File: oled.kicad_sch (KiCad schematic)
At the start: 1 part, among them J15 HC-SR04 connector

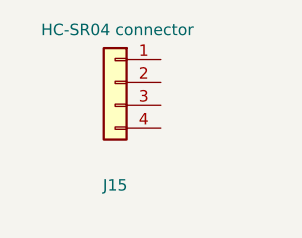
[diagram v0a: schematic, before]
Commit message: No Errors No Warnings
Some were excluded.
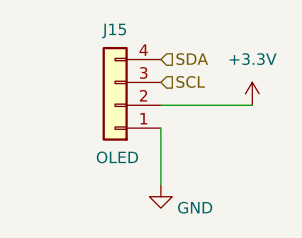
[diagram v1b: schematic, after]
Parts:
- J15: value HC-SR04 connector -> OLED; footprint Connector_PinHeader_2.54mm:PinHeader_1x04_P2.54mm_Vertical -> Connector_PinSocket_2.54mm:PinSocket_1x04_P2.54mm_Vertical
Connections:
- net GND: now reaches J15.1 (Pin_1)
- net +3.3V: now reaches J15.2 (Pin_2)
- net SCL: now reaches J15.3 (Pin_3)
- net SDA: now reaches J15.4 (Pin_4)
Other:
- moved on the sheet: J15
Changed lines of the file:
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@@
 	(generator_version "9.0")
 	(paper "A4")
+	(wire
+		(pts
+			(xy 134.62 80.01) (xy 134.62 86.36)
+		)
+		(stroke
+			(width 0)
+			(type default)
+		)
+	)
+	(wire
+		(pts
+			(xy 134.62 77.47) (xy 144.78 77.47)
+		)
+		(stroke
+			(width 0)
+			(type default)
+		)
+	)
+	(hierarchical_label "SDA"
+		(shape input)
+		(at 134.62 72.39 0)
+		(effects
+			(font
+				(size 1.27 1.27)
+			)
+			(justify left)
+		)
+	)
+	(hierarchical_label "SCL"
+		(shape input)
+		(at 134.62 74.93 0)
+		(effects
+			(font
+				(size 1.27 1.27)
+			)
+			(justify left)
+		)
+	)
+	(symbol
+		(lib_id "power:GND")
+		(at 134.62 86.36 0)
+		(unit 1)
+		(exclude_from_sim no)
+		(in_bom yes)
+		(on_board yes)
+		(dnp no)
+		(property "Reference" "#PWR0142"
+			(at 134.62 92.71 0)
+			(effects
+				(font
+					(size 1.27 1.27)
+				)
+				(hide yes)
+			)
+		)
+		(property "Value" "GND"
+			(at 138.43 88.9 0)
+			(effects
+				(font
+					(size 1.27 1.27)
+				)
+			)
+		)
+		(property "Footprint" ""
+			(at 134.62 86.36 0)
+			(effects
+				(font
+					(size 1.27 1.27)
+				)
+				(hide yes)
+			)
+		)
+		(property "Datasheet" ""
+			(at 134.62 86.36 0)
+			(effects
+				(font
+					(size 1.27 1.27)
+				)
+				(hide yes)
+			)
+		)
+		(property "Description" ""
+			(at 134.62 86.36 0)
+			(effects
+				(font
+					(size 1.27 1.27)
+				)
+				(hide yes)
+			)
+		)
+		(pin "1"
+		)
+		(instances
+			(project "Intro-to-CAD-2026"
+				(path "/c12dc015-e6cb-468c-8de4-269c3106de0e/77c9a60d-65a0-419f-902e-4b4a89f0d425"
+					(reference "#PWR0142")
+					(unit 1)
+				)
+			)
+		)
+	)
 	(symbol
 		(lib_id "Connector_Generic:Conn_01x04")
-		(at 129.54 74.93 0)
+		(at 129.54 77.47 180)
+		(unit 1)
+		(exclude_from_sim no)
+		(in_bom yes)
+		(on_board yes)
+		(dnp no)
+		(property "Reference" "J15"
+			(at 129.54 69.088 0)
+			(effects
+				(font
+					(size 1.27 1.27)
+				)
+			)
+		)
+		(property "Value" "OLED"
+			(at 129.794 83.312 0)
+			(effects
+				(font
+					(size 1.27 1.27)
+				)
+			)
+		)
+		(property "Footprint" "Connector_PinSocket_2.54mm:PinSocket_1x04_P2.54mm_Vertical"
+			(at 129.54 77.47 0)
+			(effects
+				(font
+					(size 1.27 1.27)
+				)
+				(hide yes)
+			)
+		)
+		(property "Datasheet" "https://www.robotshop.com/products/adeept-096in-oled-module-128x64-ssd1306-i2c-serial-self-luminous-display-4x?srsltid=AfmBOopotbcFOdiYSAv3nbip_y2fRyMvjxpTrSpnZLL8r5jh1ATbT-r4"
+			(at 129.54 77.47 0)
+			(effects
+				(font
+					(size 1.27 1.27)
+				)
+				(hide yes)
+			)
+		)
+		(property "Description" "Generic connector, single row, 01x04, script generated (kicad-library-utils/schlib/autogen/connector/)"
+			(at 129.54 77.47 0)
+			(effects
+				(font
+					(size 1.27 1.27)
+				)
+				(hide yes)
+			)
+		)
+		(pin "4"
+		)
+		(pin "1"
+		)
+		(pin "2"
+		)
+		(pin "3"
+		)
+		(instances
+			(project "Intro-to-CAD-2026"
+				(path "/c12dc015-e6cb-468c-8de4-269c3106de0e/77c9a60d-65a0-419f-902e-4b4a89f0d425"
+					(reference "J15")
+					(unit 1)
+				)
+			)
+		)
+	)
+	(symbol
+		(lib_id "power:+3.3V")
+		(at 144.78 77.47 0)
 		(mirror y)
 		(unit 1)
@@
 		(on_board yes)
 		(dnp no)
-		(property "Reference" "J15"
-			(at 129.54 86.36 0)
-			(effects
-				(font
-					(size 1.27 1.27)
-				)
-			)
-		)
-		(property "Value" "HC-SR04 connector"
-			(at 129.794 69.088 0)
-			(effects
-				(font
-					(size 1.27 1.27)
-				)
-			)
-		)
-		(property "Footprint" "Connector_PinHeader_2.54mm:PinHeader_1x04_P2.54mm_Vertical"
-			(at 129.54 74.93 0)
-			(effects
-				(font
-					(size 1.27 1.27)
-				)
-				(hide yes)
-			)
-		)
-		(property "Datasheet" "~"
-			(at 129.54 74.93 0)
-			(effects
-				(font
-					(size 1.27 1.27)
-				)
-				(hide yes)
-			)
-		)
-		(property "Description" "Generic connector, single row, 01x04, script generated (kicad-library-utils/schlib/autogen/connector/)"
-			(at 129.54 74.93 0)
-			(effects
-				(font
-					(size 1.27 1.27)
-				)
-				(hide yes)
-			)
-		)
-		(pin "4"
+		(fields_autoplaced yes)
+		(property "Reference" "#PWR0141"
+			(at 144.78 81.28 0)
+			(effects
+				(font
+					(size 1.27 1.27)
+				)
+				(hide yes)
+			)
+		)
+		(property "Value" "+3.3V"
+			(at 144.78 72.39 0)
+			(effects
+				(font
+					(size 1.27 1.27)
+				)
+			)
+		)
+		(property "Footprint" ""
+			(at 144.78 77.47 0)
+			(effects
+				(font
+					(size 1.27 1.27)
+				)
+				(hide yes)
+			)
+		)
+		(property "Datasheet" ""
+			(at 144.78 77.47 0)
+			(effects
+				(font
+					(size 1.27 1.27)
+				)
+				(hide yes)
+			)
+		)
+		(property "Description" ""
+			(at 144.78 77.47 0)
+			(effects
+				(font
+					(size 1.27 1.27)
+				)
+				(hide yes)
+			)
 		)
 		(pin "1"
-		)
-		(pin "2"
-		)
-		(pin "3"
 		)
 		(instances
 			(project "Intro-to-CAD-2026"
 				(path "/c12dc015-e6cb-468c-8de4-269c3106de0e/77c9a60d-65a0-419f-902e-4b4a89f0d425"
-					(reference "J15")
+					(reference "#PWR0141")
 					(unit 1)
 				)

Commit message: Getting JLCPCB Price
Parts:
- J15: LCSC (none) -> C2718488
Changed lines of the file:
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@@
+			)
+		)
+		(property "LCSC" "C2718488"
+			(at 129.54 77.47 0)
+			(effects
+				(font
+					(size 1.27 1.27)
+				)
+				(hide yes)
 			)
 		)
